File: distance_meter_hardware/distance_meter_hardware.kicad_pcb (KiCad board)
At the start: 2 copper layers, 58.4 x 58.4 mm, 6 parts, among them J1 PPPC071LFBN-RC, J2 PPPC071LFBN-RC, J3 PPPC141LFBN-RC, J4 PPPC141LFBN-RC, J5 PPPC071LFBN-RC, J6 PPPC071LFBN-RC

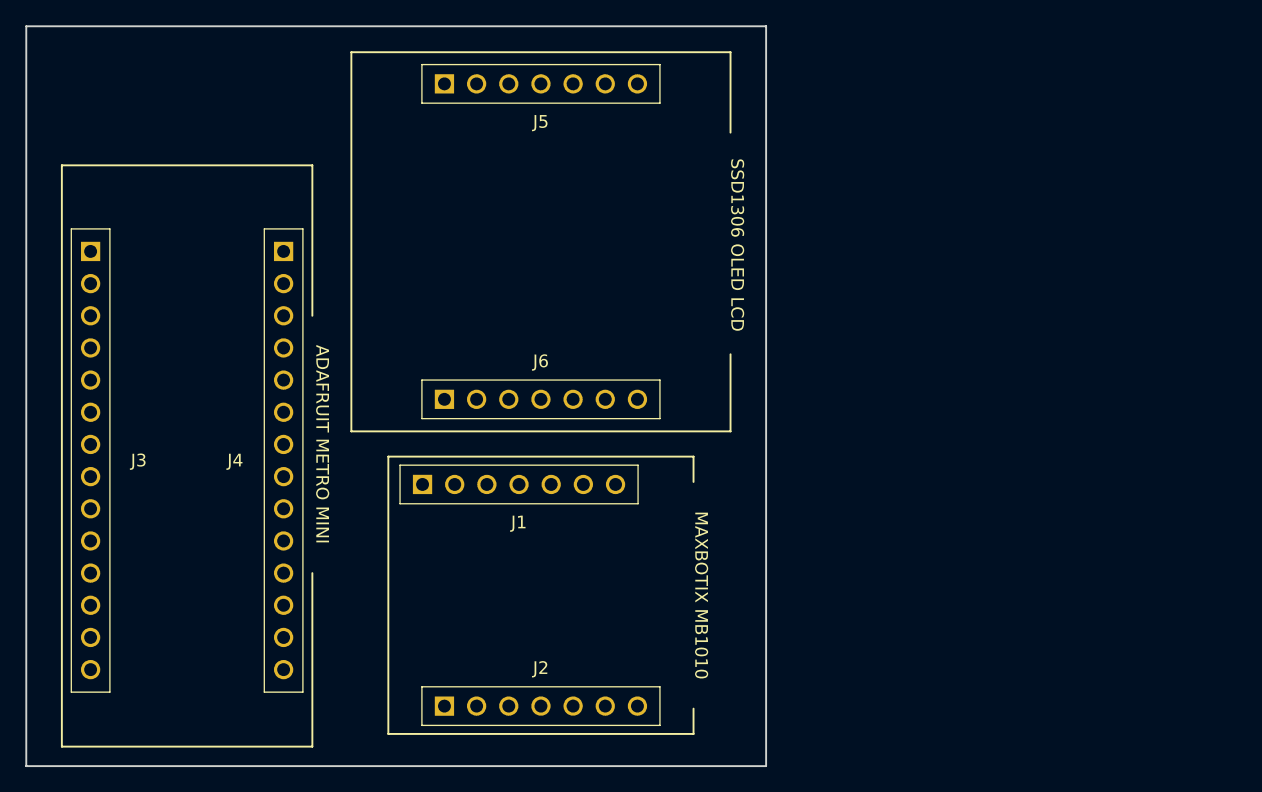
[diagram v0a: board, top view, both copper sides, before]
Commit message: Resize layout to fit in project box
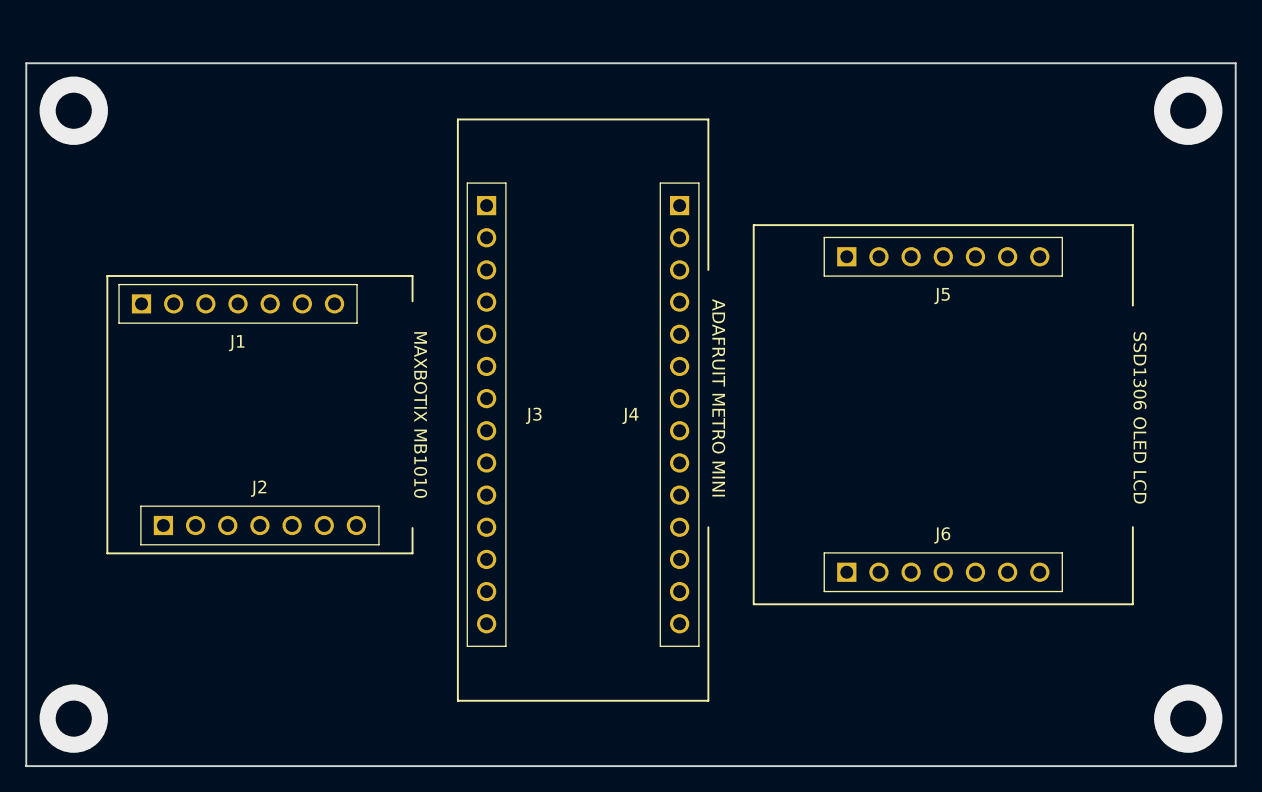
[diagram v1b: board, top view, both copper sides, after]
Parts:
- moved J5 34.6 mm to (130.8, 56.3)
- moved J6 34.6 mm to (130.8, 81.2)
- moved J4 31.5 mm to (110.0, 68.8)
- moved J3 31.5 mm to (94.8, 68.8)
- moved J1 26.4 mm to (75.1, 60.0)
- moved J2 26.4 mm to (76.9, 77.5)
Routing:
- net (no net): vias 0 -> 4
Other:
- board size 58.4 x 58.4 mm -> 95.5 x 55.5 mm
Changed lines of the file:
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@@
   (general
     (thickness 1.6)
-    (drawings 25)
-    (tracks 0)
+    (drawings 27)
+    (tracks 4)
     (zones 0)
     (modules 6)
@@
     (solder_mask_min_width 0.25)
     (aux_axis_origin 0 0)
+    (grid_origin 58.42 96.52)
     (visible_elements FFFDFF7F)
     (pcbplotparams
@@
   )
   (module headers:PPPC071LFBN-RC (layer F.Cu)
-    (at 97.33 74.280005)
+    (at 75.14 60.020005)
     (descr "http://www.sullinscorp.com/drawings/78_P(N)PxCxxxLFBN-RC,_10492-H.pdf")
     (tags "header, 1x7, socket")
@@
   )
   (module headers:PPPC071LFBN-RC (layer F.Cu)
-    (at 99.06 91.780005)
+    (at 76.87 77.520005)
     (descr "http://www.sullinscorp.com/drawings/78_P(N)PxCxxxLFBN-RC,_10492-H.pdf")
     (tags "header, 1x7, socket")
@@
   )
   (module headers:PPPC141LFBN-RC (layer F.Cu)
-    (at 63.5 72.39 270)
+    (at 94.77 68.77 270)
     (descr "http://www.sullinscorp.com/drawings/78_P(N)PxCxxxLFBN-RC,_10492-H.pdf")
     (tags "header, 1x14, socket")
@@
   )
   (module headers:PPPC141LFBN-RC (layer F.Cu)
-    (at 78.74 72.39 270)
+    (at 110.01 68.77 270)
     (descr "http://www.sullinscorp.com/drawings/78_P(N)PxCxxxLFBN-RC,_10492-H.pdf")
     (tags "header, 1x14, socket")
@@
   )
   (module headers:PPPC071LFBN-RC (layer F.Cu)
-    (at 99.06 42.648)
+    (at 130.83 56.3)
     (descr "http://www.sullinscorp.com/drawings/78_P(N)PxCxxxLFBN-RC,_10492-H.pdf")
     (tags "header, 1x7, socket")
@@
   )
   (module headers:PPPC071LFBN-RC (layer F.Cu)
-    (at 99.06 67.558)
+    (at 130.83 81.21)
     (descr "http://www.sullinscorp.com/drawings/78_P(N)PxCxxxLFBN-RC,_10492-H.pdf")
     (tags "header, 1x7, socket")
@@
     )
   )
-  (gr_poly (pts (xy 62.23 50.8) (xy 80.01 50.8) (xy 80.01 93.98) (xy 62.23 93.98)) (layer F.Fab) (width 0.1))
-  (gr_text "SSD1306 OLED LCD" (at 114.554 55.372 270) (layer F.SilkS)
+  (dimension 55.5 (width 0.15) (layer F.SilkS)
+    (gr_text "55.500 mm" (at 40.12 68.77 90) (layer F.SilkS)
+      (effects (font (size 1 1) (thickness 0.15)))
+    )
+    (feature1 (pts (xy 58.42 41.02) (xy 40.833579 41.02)))
+    (feature2 (pts (xy 58.42 96.52) (xy 40.833579 96.52)))
+    (crossbar (pts (xy 41.42 96.52) (xy 41.42 41.02)))
+    (arrow1a (pts (xy 41.42 41.02) (xy 42.006421 42.146504)))
+    (arrow1b (pts (xy 41.42 41.02) (xy 40.833579 42.146504)))
+    (arrow2a (pts (xy 41.42 96.52) (xy 42.006421 95.393496)))
+    (arrow2b (pts (xy 41.42 96.52) (xy 40.833579 95.393496)))
+  )
+  (dimension 95.5 (width 0.15) (layer F.SilkS)
+    (gr_text "95.500 mm" (at 106.17 103.32) (layer F.SilkS)
+      (effects (font (size 1 1) (thickness 0.15)))
+    )
+    (feature1 (pts (xy 153.92 96.52) (xy 153.92 102.606421)))
+    (feature2 (pts (xy 58.42 96.52) (xy 58.42 102.606421)))
+    (crossbar (pts (xy 58.42 102.02) (xy 153.92 102.02)))
+    (arrow1a (pts (xy 153.92 102.02) (xy 152.793496 102.606421)))
+    (arrow1b (pts (xy 153.92 102.02) (xy 152.793496 101.433579)))
+    (arrow2a (pts (xy 58.42 102.02) (xy 59.546504 102.606421)))
+    (arrow2b (pts (xy 58.42 102.02) (xy 59.546504 101.433579)))
+  )
+  (gr_poly (pts (xy 93.5 47.18) (xy 111.28 47.18) (xy 111.28 90.36) (xy 93.5 90.36)) (layer F.Fab) (width 0.1))
+  (gr_text "SSD1306 OLED LCD" (at 146.324 69.024 270) (layer F.SilkS)
     (effects (font (size 1 1) (thickness 0.15)))
   )
-  (gr_line (start 114.03 70.088) (end 114.03 64) (layer F.SilkS) (width 0.15))
-  (gr_line (start 84.09 70.088) (end 114.03 70.088) (layer F.SilkS) (width 0.15))
-  (gr_line (start 84.09 40.148) (end 84.09 70.088) (layer F.SilkS) (width 0.15))
-  (gr_line (start 114.03 40.148) (end 114.03 46.5) (layer F.SilkS) (width 0.15))
-  (gr_line (start 84.09 40.148) (end 114.03 40.148) (layer F.SilkS) (width 0.15))
-  (gr_poly (pts (xy 85.09 41.148) (xy 113.03 41.148) (xy 113.03 69.088) (xy 85.09 69.088)) (layer F.Fab) (width 0.1))
-  (gr_poly (pts (xy 88.01 73.080005) (xy 110.11 73.080005) (xy 110.11 92.980005) (xy 88.01 92.980005)) (layer F.Fab) (width 0.1))
-  (gr_line (start 111.11 93.980005) (end 111.11 91.980005) (layer F.SilkS) (width 0.15))
-  (gr_line (start 111.11 72.080005) (end 111.11 74.080005) (layer F.SilkS) (width 0.15))
-  (gr_text "MAXBOTIX MB1010" (at 111.71 83.030005 270) (layer F.SilkS)
+  (gr_line (start 145.8 83.74) (end 145.8 77.652) (layer F.SilkS) (width 0.15))
+  (gr_line (start 115.86 83.74) (end 145.8 83.74) (layer F.SilkS) (width 0.15))
+  (gr_line (start 115.86 53.8) (end 115.86 83.74) (layer F.SilkS) (width 0.15))
+  (gr_line (start 145.8 53.8) (end 145.8 60.152) (layer F.SilkS) (width 0.15))
+  (gr_line (start 115.86 53.8) (end 145.8 53.8) (layer F.SilkS) (width 0.15))
+  (gr_poly (pts (xy 116.86 54.8) (xy 144.8 54.8) (xy 144.8 82.74) (xy 116.86 82.74)) (layer F.Fab) (width 0.1))
+  (gr_poly (pts (xy 65.82 58.820005) (xy 87.92 58.820005) (xy 87.92 78.720005) (xy 65.82 78.720005)) (layer F.Fab) (width 0.1))
+  (gr_line (start 88.92 79.720005) (end 88.92 77.720005) (layer F.SilkS) (width 0.15))
+  (gr_line (start 88.92 57.820005) (end 88.92 59.820005) (layer F.SilkS) (width 0.15))
+  (gr_text "MAXBOTIX MB1010" (at 89.52 68.770005 270) (layer F.SilkS)
     (effects (font (size 1 1) (thickness 0.15)))
   )
-  (gr_line (start 87.01 93.980005) (end 87.01 72.080005) (layer F.SilkS) (width 0.15))
-  (gr_line (start 111.11 93.980005) (end 87.01 93.980005) (layer F.SilkS) (width 0.15))
-  (gr_line (start 87.01 72.080005) (end 111.11 72.080005) (layer F.SilkS) (width 0.15))
-  (gr_line (start 81.01 94.98) (end 81.01 81.28) (layer F.SilkS) (width 0.15))
-  (gr_line (start 81.01 49.08) (end 81.01 60.96) (layer F.SilkS) (width 0.15))
-  (gr_text "ADAFRUIT METRO MINI" (at 81.788 71.12 270) (layer F.SilkS)
+  (gr_line (start 64.82 79.720005) (end 64.82 57.820005) (layer F.SilkS) (width 0.15))
+  (gr_line (start 88.92 79.720005) (end 64.82 79.720005) (layer F.SilkS) (width 0.15))
+  (gr_line (start 64.82 57.820005) (end 88.92 57.820005) (layer F.SilkS) (width 0.15))
+  (gr_line (start 112.28 91.36) (end 112.28 77.66) (layer F.SilkS) (width 0.15))
+  (gr_line (start 112.28 45.46) (end 112.28 57.34) (layer F.SilkS) (width 0.15))
+  (gr_text "ADAFRUIT METRO MINI" (at 113.058 67.5 270) (layer F.SilkS)
     (effects (font (size 1 1) (thickness 0.15)))
   )
-  (gr_line (start 61.23 94.98) (end 81.01 94.98) (layer F.SilkS) (width 0.15))
-  (gr_line (start 61.23 49.08) (end 61.23 94.98) (layer F.SilkS) (width 0.15))
-  (gr_line (start 61.23 49.08) (end 81.01 49.08) (layer F.SilkS) (width 0.15))
-  (gr_line (start 58.42 96.52) (end 58.42 38.1) (layer Edge.Cuts) (width 0.15))
-  (gr_line (start 116.84 96.52) (end 58.42 96.52) (layer Edge.Cuts) (width 0.15))
-  (gr_line (start 116.84 38.1) (end 116.84 96.52) (layer Edge.Cuts) (width 0.15))
-  (gr_line (start 58.42 38.1) (end 116.84 38.1) (layer Edge.Cuts) (width 0.15))
+  (gr_line (start 92.5 91.36) (end 112.28 91.36) (layer F.SilkS) (width 0.15))
+  (gr_line (start 92.5 45.46) (end 92.5 91.36) (layer F.SilkS) (width 0.15))
+  (gr_line (start 92.5 45.46) (end 112.28 45.46) (layer F.SilkS) (width 0.15))
+  (gr_line (start 58.42 96.52) (end 58.42 41.02) (layer Edge.Cuts) (width 0.15))
+  (gr_line (start 153.92 96.52) (end 58.42 96.52) (layer Edge.Cuts) (width 0.15))
+  (gr_line (start 153.92 41.02) (end 153.92 96.52) (layer Edge.Cuts) (width 0.15))
+  (gr_line (start 58.42 41.02) (end 153.92 41.02) (layer Edge.Cuts) (width 0.15))
+  (via (at 150.17 44.77) (size 5.4) (drill 2.85) (layers F.Cu B.Cu) (net 0))
+  (via (at 150.17 92.77) (size 5.4) (drill 2.85) (layers F.Cu B.Cu) (net 0))
+  (via (at 62.17 92.77) (size 5.4) (drill 2.85) (layers F.Cu B.Cu) (net 0))
+  (via (at 62.17 44.77) (size 5.4) (drill 2.85) (layers F.Cu B.Cu) (net 0))
 )
